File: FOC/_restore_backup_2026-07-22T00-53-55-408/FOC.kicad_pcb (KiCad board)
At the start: 4 copper layers, 79 x 34.9 mm, 74 parts, among them J1 encoder_conn, J2 Conn_ARM_JTAG_SWD_10, J3 UART_debug, J4 XT30PW-M, J5 Conn_01x04_Socket, J6 Conn_01x04_Socket, J7 Conn_01x03_Socket, SW1 SW_Push, SW2 SW_Push, U1 STM32G431CBTx, U2 SN65HVD230, U3 TPS54202DDC, U4 AP2112K-3.3, U5 DRV8313PWP, Y1 Crystal_GND24

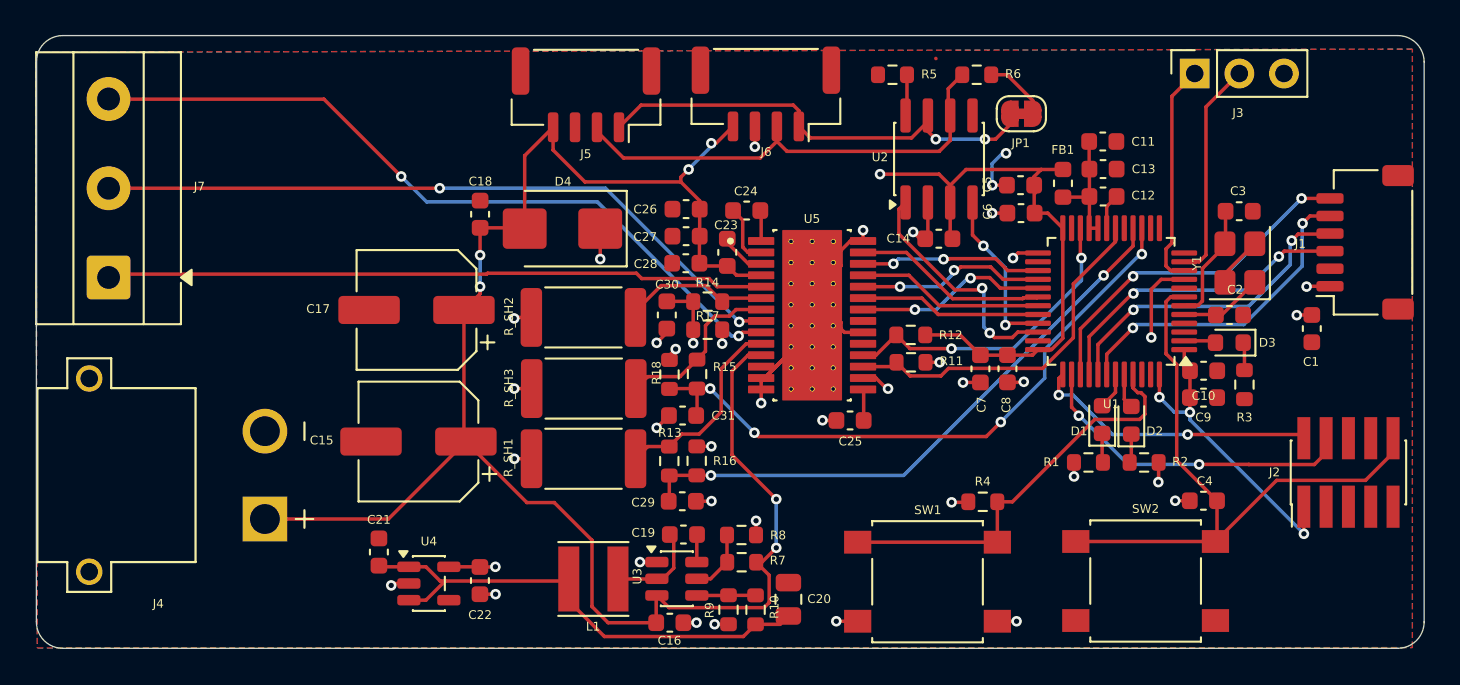
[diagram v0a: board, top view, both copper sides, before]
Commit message: four layer pour; layout done
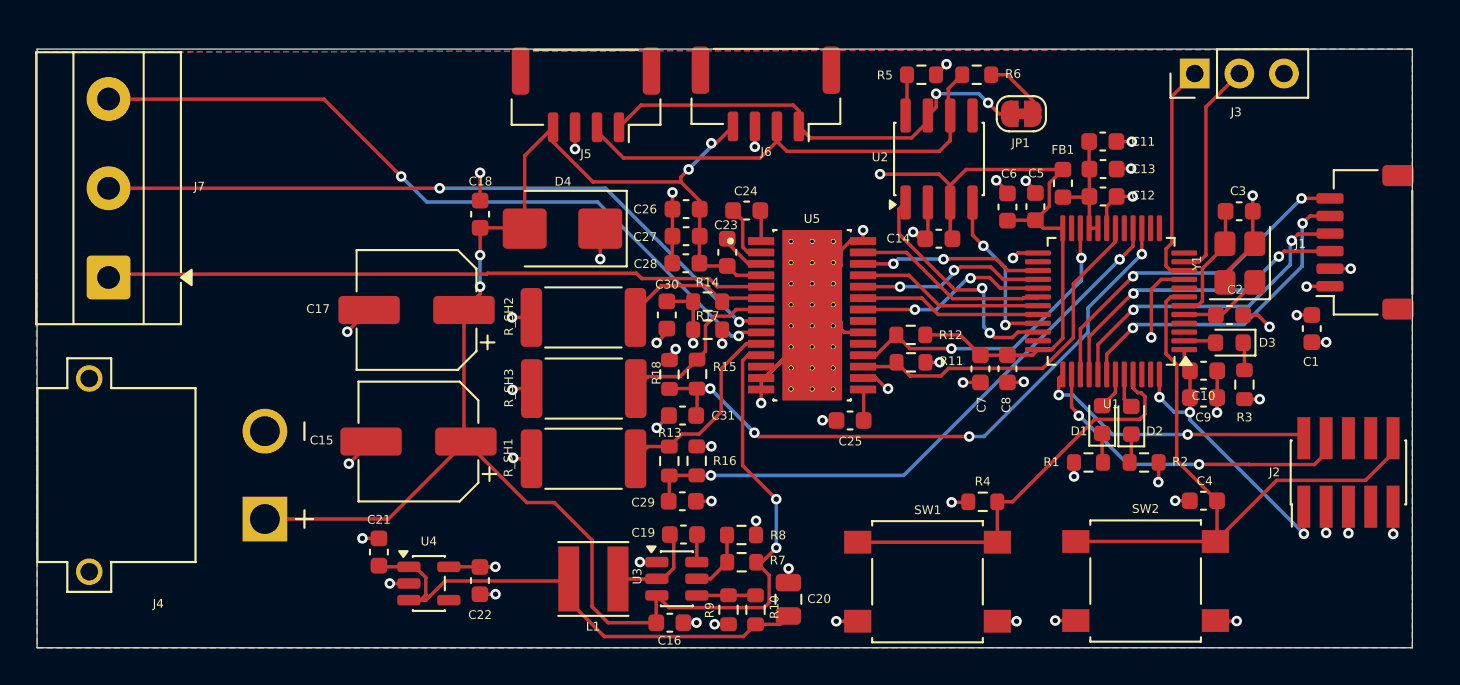
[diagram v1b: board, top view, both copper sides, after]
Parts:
- J3: footprint Connector_PinSocket_2.54mm:PinSocket_1x03_P2.54mm_Vertical -> Connector_PinHeader_2.54mm:PinHeader_1x03_P2.54mm_Vertical
- moved R5 1.65 mm to (131.0, 38.1), turned to 0 degrees
- moved C5 1.48 mm to (137.5, 45.6), turned to -90 degrees
- moved C6 0.84 mm to (135.9, 45.7), turned to -90 degrees
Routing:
- net GND: track 58.1 -> 88.7 mm, vias 28 -> 49
- net +3.3V: track 75.5 -> 77.7 mm
- net +5V: track 28.8 -> 29.7 mm
- net VM: track 100.5 -> 99.7 mm
- net CANH: track 26.9 -> 26.2 mm
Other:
- board size 79 x 34.9 mm -> 78.3 x 34.1 mm
